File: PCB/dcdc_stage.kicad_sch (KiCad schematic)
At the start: 0 parts

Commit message: esp32 various fix, 20to3v3 DCDC.
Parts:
- added C14: 4u7 50V 0805 X7R, symbol Device:C
- added C15: 22pF 50V C0G 0402, symbol Device:C
- added C16: 22uF 0805 10V X7R, symbol Device:C
- added C17: 100nF 50V X7R 0402, symbol Device:C
- added IC4: MPM3510AGQV, QFN-19, symbol SamacSys_Parts:MPM3510AGQV-P
- added NT3: NetTie_2, Jumper:SolderJumper-2_P1.3mm_Bridged_Pad1.0x1.5mm, symbol Device:NetTie_2
- added R24: 100K 0402 5% 62.5mW, symbol Device:R
- added R25: 75K 0402 1% 62.5mW, symbol Device:R
- added R26: 24K 0402 1% 62.5mW, symbol Device:R
- added R27: 1M 0402 5% 62.5mW, symbol Device:R
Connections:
- new net: C15.2, IC4.1 (FB), R25.2, R26.1
- new net: IC4.16 (EN/SYNC), R27.2
- new net +3V3: R24.2
- new net GND: C14.2, C16.2, C17.2, IC4.12 (PGND_1), IC4.13 (PGND_2), IC4.3 (AGND), NT3.2, R26.2
- new net GNDA: NT3.1
- new net PG_OUT: IC4.17 (PG), R24.1
- new net VIN: C14.1, C17.1, IC4.15 (IN), R27.1
- new net VOUT_3V3: C15.1, C16.1, IC4.7 (OUT_1), IC4.8 (OUT_2), IC4.9 (OUT_3), R25.1
- no-connect marks 0 -> 7
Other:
- note added: "Switch output. No connection is needed for the SW pins, but a large copper plane is recommended on pins 4, 5, and 6 to improve heat sink"

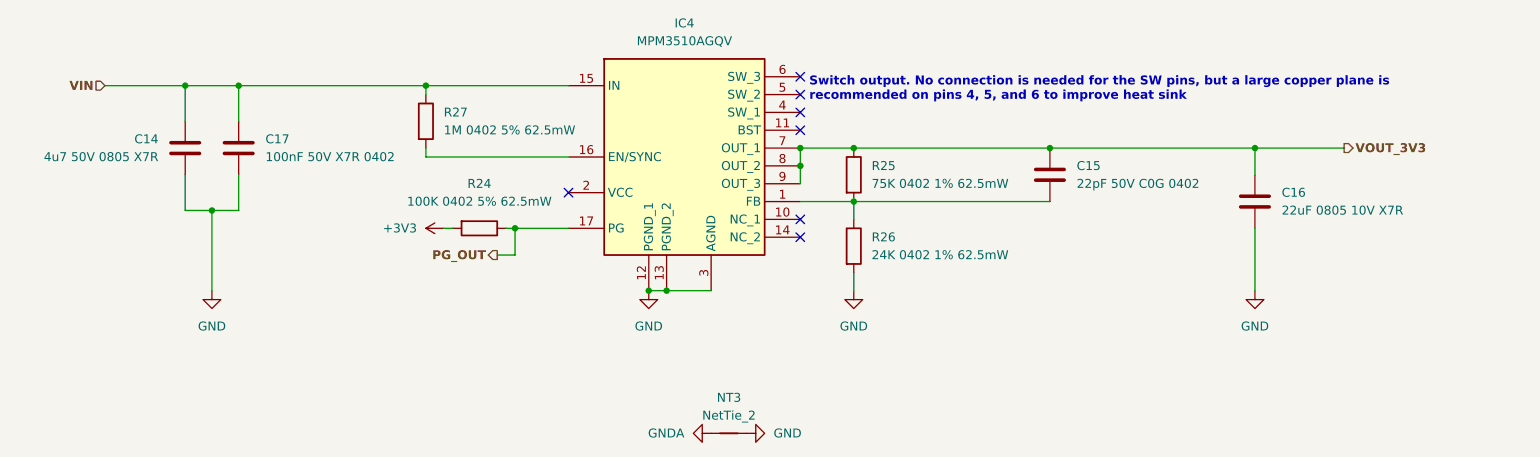
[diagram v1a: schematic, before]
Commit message: stusb schematic
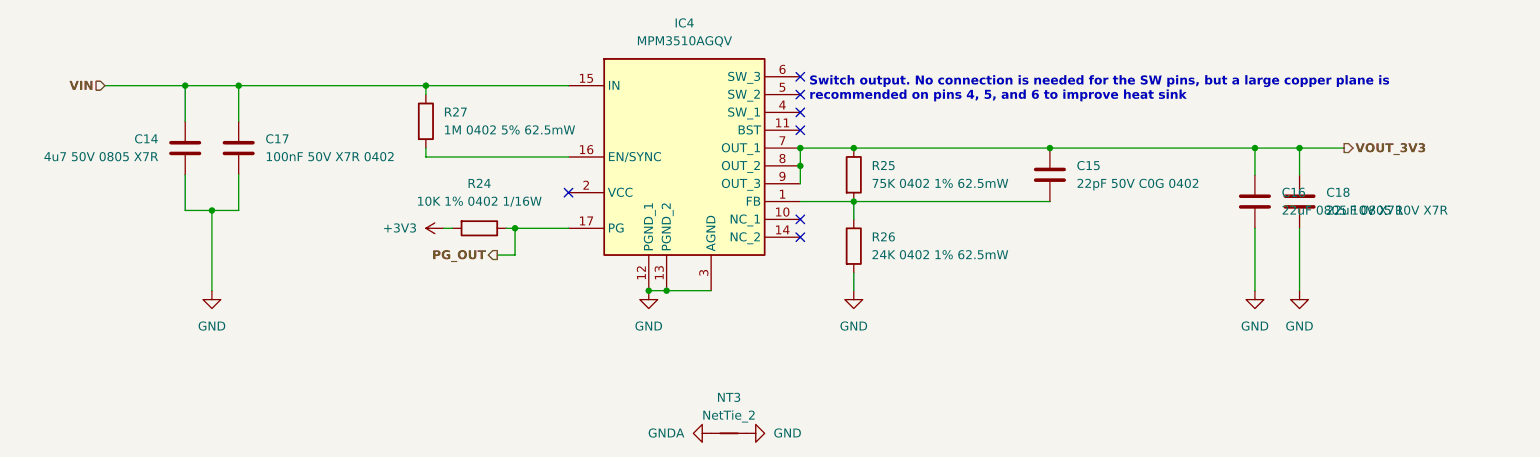
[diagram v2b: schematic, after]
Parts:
- added C18: 22uF 0805 10V X7R, Capacitor_SMD:C_0805_2012Metric_Pad1.18x1.45mm_HandSolder, symbol Device:C
- C14, C16: footprint (none) -> Capacitor_SMD:C_0805_2012Metric_Pad1.18x1.45mm_HandSolder
- C15, C17, R25, R26, R27: footprint (none) -> Capacitor_SMD:C_0402_1005Metric_Pad0.74x0.62mm_HandSolder
- IC4: footprint QFN-19 -> SamacSys_Parts:QFN-19
- R24: value 100K 0402 5% 62.5mW -> 10K 1% 0402 1/16W; footprint (none) -> Resistor_SMD:R_0402_1005Metric_Pad0.72x0.64mm_HandSolder; MPN RC0402JR-07100KL -> RC0402FR-0710KL
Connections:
- net GND: now also C18.2
- net VOUT_3V3: now also C18.1
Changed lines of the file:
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@@
+	)
+	(junction
+		(at 199.39 77.47)
+		(diameter 0)
+		(color 0 0 0 0)
 	)
 	(junction
@@
 	(wire
 		(pts
+			(xy 199.39 97.79) (xy 199.39 88.9)
+		)
+		(stroke
+			(width 0)
+			(type default)
+		)
+	)
+	(wire
+		(pts
 			(xy 85.09 92.71) (xy 87.63 92.71)
 		)
@@
 	(wire
 		(pts
-			(xy 193.04 77.47) (xy 205.74 77.47)
+			(xy 193.04 77.47) (xy 199.39 77.47)
 		)
 		(stroke
@@
 	(wire
 		(pts
+			(xy 199.39 81.28) (xy 199.39 77.47)
+		)
+		(stroke
+			(width 0)
+			(type default)
+		)
+	)
+	(wire
+		(pts
 			(xy 135.89 87.63) (xy 135.89 85.09)
 		)
@@
 		(pts
 			(xy 128.27 77.47) (xy 135.89 77.47)
+		)
+		(stroke
+			(width 0)
+			(type default)
+		)
+	)
+	(wire
+		(pts
+			(xy 199.39 77.47) (xy 205.74 77.47)
 		)
 		(stroke
@@
 	)
 	(symbol
+		(lib_id "Device:C")
+		(at 199.39 85.09 0)
+		(unit 1)
+		(exclude_from_sim no)
+		(in_bom yes)
+		(on_board yes)
+		(dnp no)
+		(fields_autoplaced yes)
+		(property "Reference" "C18"
+			(at 203.2 83.8199 0)
+			(effects
+				(font
+					(size 1.27 1.27)
+				)
+				(justify left)
+			)
+		)
+		(property "Value" "22uF 0805 10V X7R"
+			(at 203.2 86.3599 0)
+			(effects
+				(font
+					(size 1.27 1.27)
+				)
+				(justify left)
+			)
+		)
+		(property "Footprint" "Capacitor_SMD:C_0805_2012Metric_Pad1.18x1.45mm_HandSolder"
+			(at 200.3552 88.9 0)
+			(effects
+				(font
+					(size 1.27 1.27)
+				)
+				(hide yes)
+			)
+		)
+		(property "Datasheet" "~"
+			(at 199.39 85.09 0)
+			(effects
+				(font
+					(size 1.27 1.27)
+				)
+				(hide yes)
+			)
+		)
+		(property "Description" "Unpolarized capacitor"
+			(at 199.39 85.09 0)
+			(effects
+				(font
+					(size 1.27 1.27)
+				)
+				(hide yes)
+			)
+		)
+		(property "MPN" "GRM21BZ71A226ME15L"
+			(at 199.39 85.09 0)
+			(effects
+				(font
+					(size 1.27 1.27)
+				)
+				(hide yes)
+			)
+		)
+		(property "Manufacturer" "muRata"
+			(at 199.39 85.09 0)
+			(effects
+				(font
+					(size 1.27 1.27)
+				)
+				(hide yes)
+			)
+		)
+		(pin "2"
+		)
+		(pin "1"
+		)
+		(instances
+			(project "PCB"
+				(path "/6bd10cb8-11ca-4919-a8d8-88b44cd4cac7/3defd80d-ca54-40d3-89df-c500ad5dd04e"
+					(reference "C18")
+					(unit 1)
+				)
+			)
+		)
+	)
+	(symbol
 		(lib_id "power:GND")
 		(at 193.04 97.79 0)
@@
 			)
 		)
-		(property "Footprint" ""
+		(property "Footprint" "Capacitor_SMD:C_0402_1005Metric_Pad0.74x0.62mm_HandSolder"
 			(at 164.7952 85.09 0)
 			(effects
@@
 			)
 		)
-		(property "Footprint" ""
+		(property "Footprint" "Capacitor_SMD:C_0402_1005Metric_Pad0.74x0.62mm_HandSolder"
 			(at 134.112 91.44 90)
 			(effects
@@
 			)
 		)
-		(property "Footprint" ""
+		(property "Footprint" "Capacitor_SMD:C_0402_1005Metric_Pad0.74x0.62mm_HandSolder"
 			(at 73.152 73.66 90)
 			(effects
@@
 			)
 		)
-		(property "Footprint" ""
+		(property "Footprint" "Capacitor_SMD:C_0805_2012Metric_Pad1.18x1.45mm_HandSolder"
 			(at 194.0052 88.9 0)
 			(effects
@@
 			)
 		)
-		(property "Footprint" ""
+		(property "Footprint" "Capacitor_SMD:C_0402_1005Metric_Pad0.74x0.62mm_HandSolder"
 			(at 49.2252 81.28 0)
 			(effects
@@
 	(symbol
 		(lib_id "Device:R")
+		(at 82.55 88.9 270)
+		(unit 1)
+		(exclude_from_sim no)
+		(in_bom yes)
+		(on_board yes)
+		(dnp no)
+		(fields_autoplaced yes)
+		(property "Reference" "R24"
+			(at 82.55 82.55 90)
+			(effects
+				(font
+					(size 1.27 1.27)
+				)
+			)
+		)
+		(property "Value" "10K 1% 0402 1/16W"
+			(at 82.55 85.09 90)
+			(effects
+				(font
+					(size 1.27 1.27)
+				)
+			)
+		)
+		(property "Footprint" "Resistor_SMD:R_0402_1005Metric_Pad0.72x0.64mm_HandSolder"
+			(at 82.55 87.122 90)
+			(effects
+				(font
+					(size 1.27 1.27)
+				)
+				(hide yes)
+			)
+		)
+		(property "Datasheet" "~"
+			(at 82.55 88.9 0)
+			(effects
+				(font
+					(size 1.27 1.27)
+				)
+				(hide yes)
+			)
+		)
+		(property "Description" "Resistor"
+			(at 82.55 88.9 0)
+			(effects
+				(font
+					(size 1.27 1.27)
+				)
+				(hide yes)
+			)
+		)
+		(property "MPN" "RC0402FR-0710KL"
+			(at 82.55 88.9 90)
+			(effects
+				(font
+					(size 1.27 1.27)
+				)
+				(hide yes)
+			)
+		)
+		(property "Manufacturer" "YAGEO"
+			(at 82.55 88.9 90)
+			(effects
+				(font
+					(size 1.27 1.27)
+				)
+				(hide yes)
+			)
+		)
+		(pin "1"
+		)
+		(pin "2"
+		)
+		(instances
+			(project "PCB"
+				(path "/6bd10cb8-11ca-4919-a8d8-88b44cd4cac7/3defd80d-ca54-40d3-89df-c500ad5dd04e"
+					(reference "R24")
+					(unit 1)
+				)
+			)
+		)
+	)
+	(symbol
+		(lib_id "Device:R")
 		(at 135.89 81.28 0)
 		(unit 1)
@@
 			)
 		)
-		(property "Footprint" ""
+		(property "Footprint" "Capacitor_SMD:C_0402_1005Metric_Pad0.74x0.62mm_HandSolder"
 			(at 134.112 81.28 90)
 			(effects
@@
 	)
 	(symbol
-		(lib_id "Device:R")
-		(at 82.55 88.9 270)
+		(lib_id "power:GND")
+		(at 199.39 97.79 0)
 		(unit 1)
 		(exclude_from_sim no)
@@
 		(dnp no)
 		(fields_autoplaced yes)
-		(property "Reference" "R24"
-			(at 82.55 82.55 90)
-			(effects
-				(font
-					(size 1.27 1.27)
-				)
-			)
-		)
-		(property "Value" "100K 0402 5% 62.5mW"
-			(at 82.55 85.09 90)
+		(property "Reference" "#PWR058"
+			(at 199.39 104.14 0)
+			(effects
+				(font
+					(size 1.27 1.27)
+				)
+				(hide yes)
+			)
+		)
+		(property "Value" "GND"
+			(at 199.39 102.87 0)
 			(effects
 				(font
@@
 		)
 		(property "Footprint" ""
-			(at 82.55 87.122 90)
-			(effects
-				(font
-					(size 1.27 1.27)
-				)
-				(hide yes)
-			)
-		)
-		(property "Datasheet" "~"
-			(at 82.55 88.9 0)
-			(effects
-				(font
-					(size 1.27 1.27)
-				)
-				(hide yes)
-			)
-		)
-		(property "Description" "Resistor"
-			(at 82.55 88.9 0)
-			(effects
-				(font
-					(size 1.27 1.27)
-				)
-				(hide yes)
-			)
-		)
-		(property "MPN" "RC0402JR-07100KL"
-			(at 82.55 88.9 90)
-			(effects
-				(font
-					(size 1.27 1.27)
-				)
-				(hide yes)
-			)
-		)
-		(property "Manufacturer" "YAGEO"
-			(at 82.55 88.9 90)
-			(effects
-				(font
-					(size 1.27 1.27)
-				)
-				(hide yes)
-			)
-		)
-		(pin "2"
+			(at 199.39 97.79 0)
+			(effects
+				(font
+					(size 1.27 1.27)
+				)
+				(hide yes)
+			)
+		)
+		(property "Datasheet" ""
+			(at 199.39 97.79 0)
+			(effects
+				(font
+					(size 1.27 1.27)
+				)
+				(hide yes)
+			)
+		)
+		(property "Description" "Power symbol creates a global label with name \"GND\" , ground"
+			(at 199.39 97.79 0)
+			(effects
+				(font
+					(size 1.27 1.27)
+				)
+				(hide yes)
+			)
 		)
 		(pin "1"
@@
 			(project "PCB"
 				(path "/6bd10cb8-11ca-4919-a8d8-88b44cd4cac7/3defd80d-ca54-40d3-89df-c500ad5dd04e"
-					(reference "R24")
+					(reference "#PWR058")
 					(unit 1)
 				)
@@
 			)
 		)
-		(property "Footprint" "QFN-19"
+		(property "Footprint" "SamacSys_Parts:QFN-19"
 			(at 140.97 173.66 0)
 			(effects
@@
 			)
 		)
-		(property "Footprint" ""
+		(property "Footprint" "Capacitor_SMD:C_0805_2012Metric_Pad1.18x1.45mm_HandSolder"
 			(at 41.6052 81.28 0)
 			(effects
